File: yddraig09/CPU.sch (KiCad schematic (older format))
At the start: 4 parts

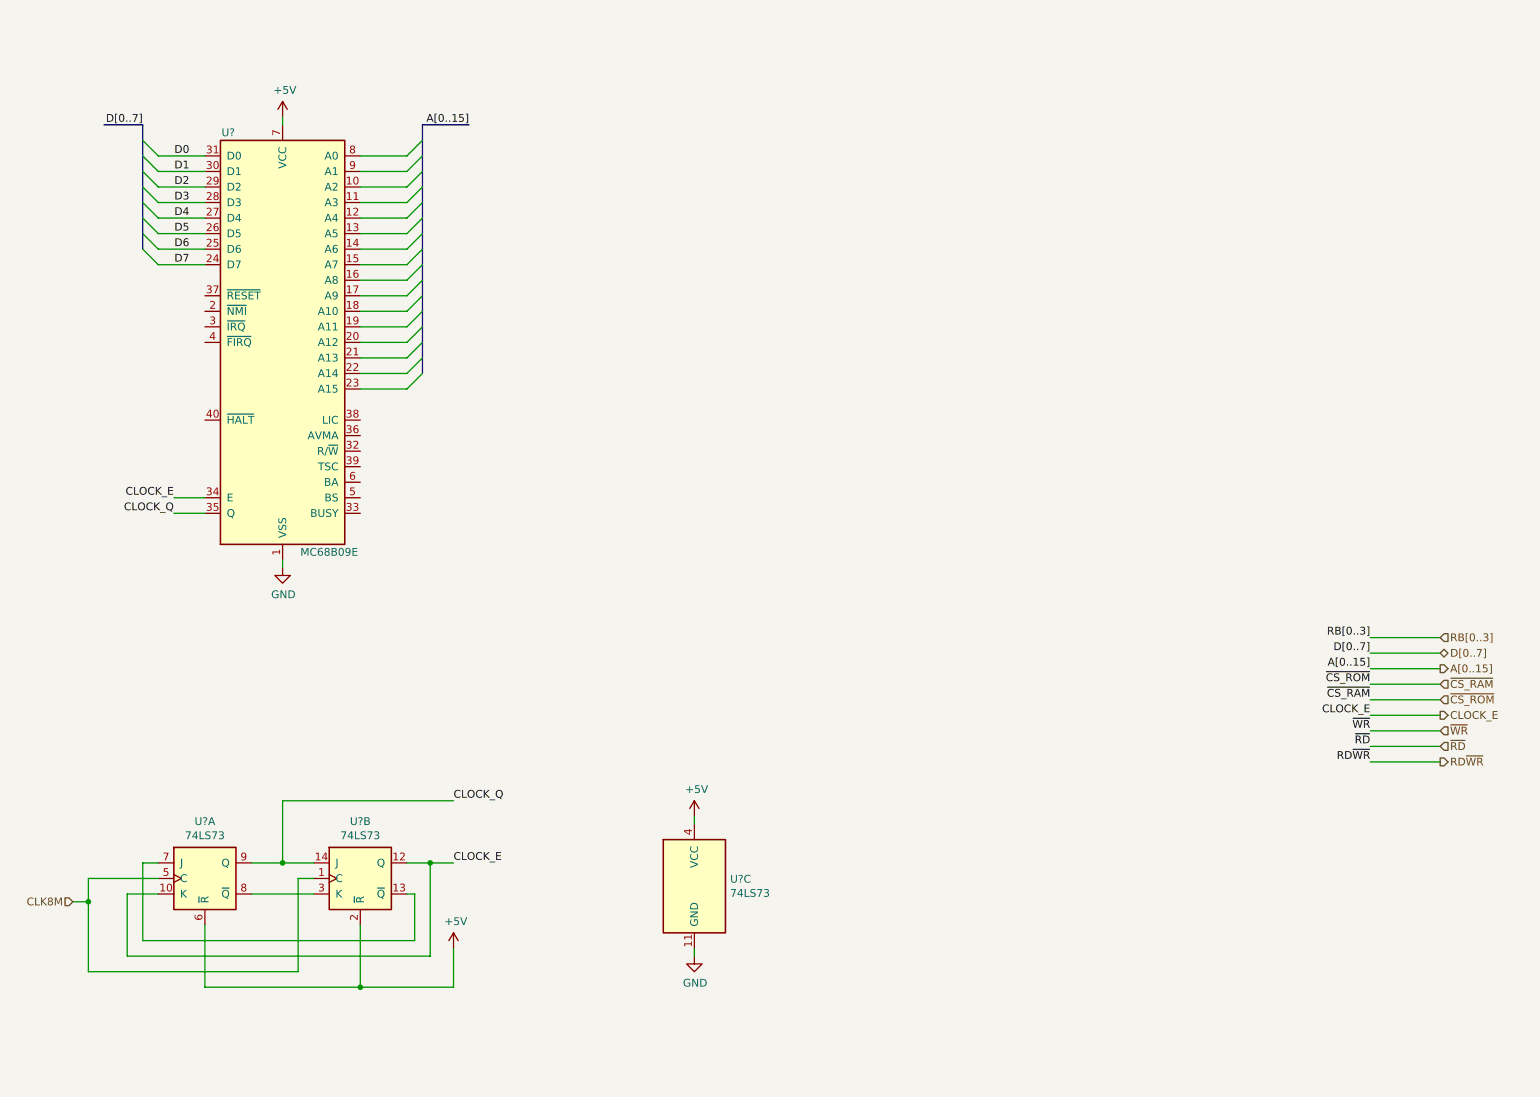
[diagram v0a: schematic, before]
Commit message: Some tidying up of 6809 project
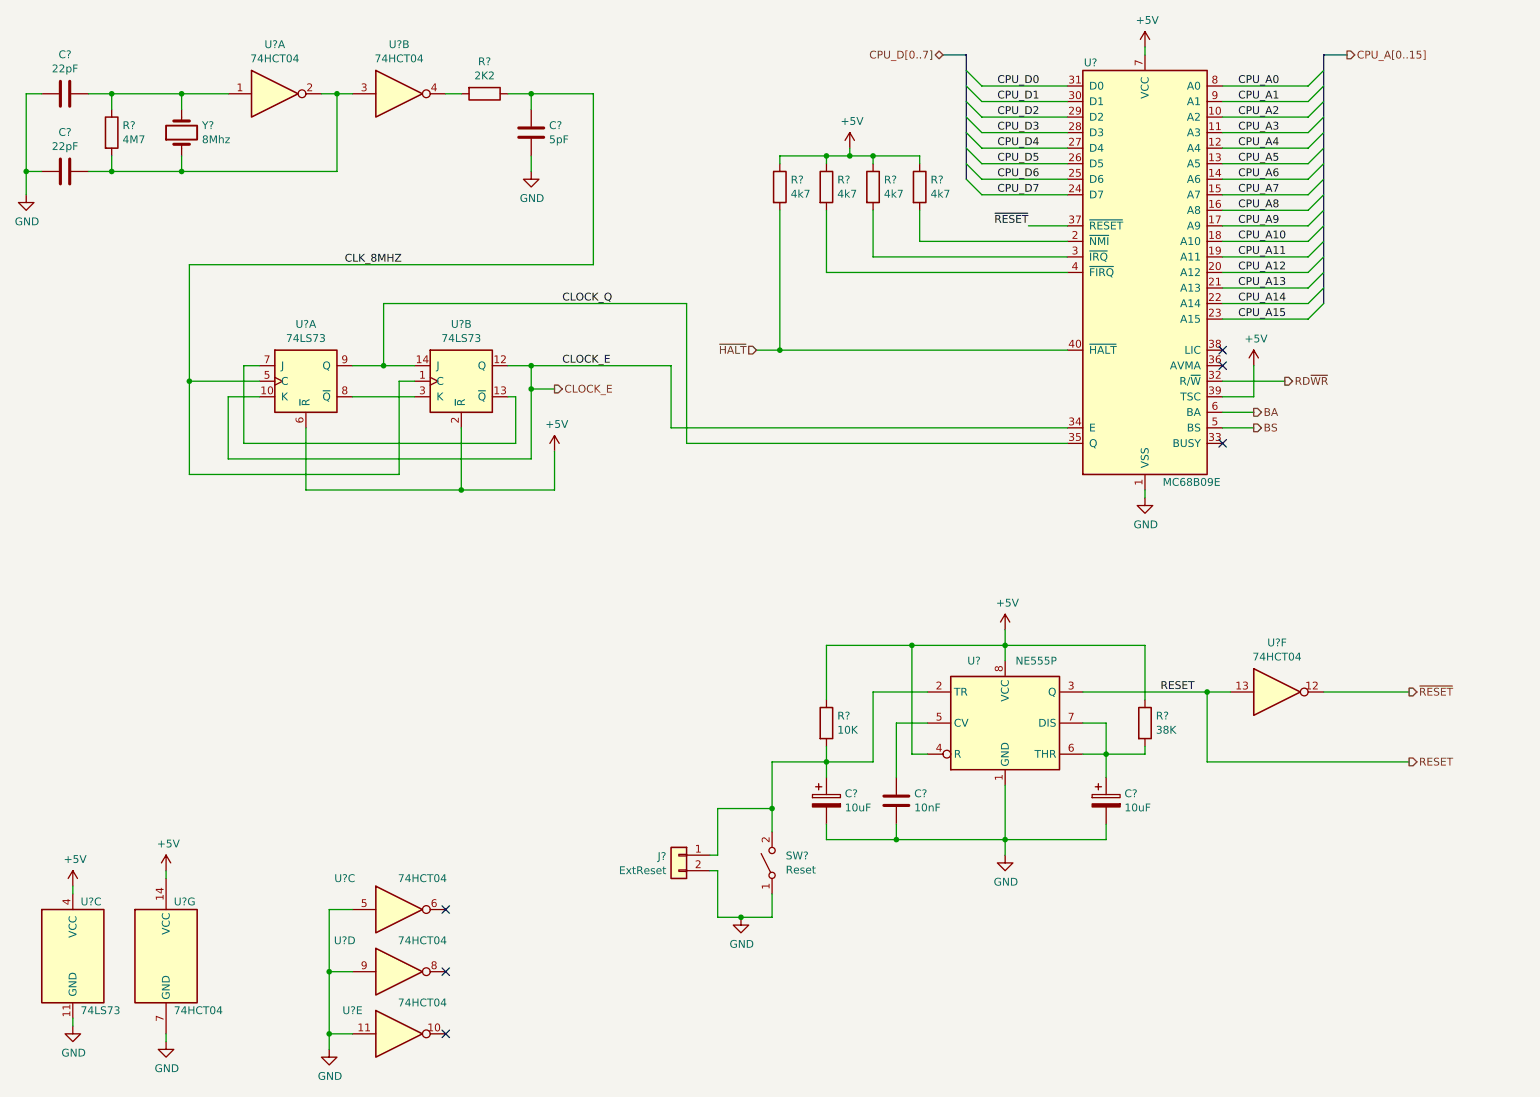
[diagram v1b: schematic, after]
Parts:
- added C? (x2): 10uF, Capacitor_THT:CP_Radial_D5.0mm_P2.50mm, symbol Device:CP
- added C?: 10nF, Capacitor_THT:C_Disc_D3.8mm_W2.6mm_P2.50mm, symbol Device:C
- added C? (x2): 22pF, Capacitor_THT:C_Disc_D5.0mm_W2.5mm_P2.50mm, symbol Device:C
- added C?: 5pF, Capacitor_THT:C_Disc_D5.0mm_W2.5mm_P2.50mm, symbol Device:C
- added J?: ExtReset, Connector_PinHeader_2.54mm:PinHeader_1x02_P2.54mm_Vertical, symbol Connector_Generic:Conn_01x02
- added R?: 10K, Resistor_THT:R_Axial_DIN0207_L6.3mm_D2.5mm_P10.16mm_Horizontal, symbol Device:R
- added R?: 38K, Resistor_THT:R_Axial_DIN0207_L6.3mm_D2.5mm_P10.16mm_Horizontal, symbol Device:R
- added R? (x4): 4k7, symbol Device:R
- added R?: 4M7, Resistor_THT:R_Axial_DIN0207_L6.3mm_D2.5mm_P10.16mm_Horizontal, symbol Device:R
- added R?: 2K2, Resistor_THT:R_Axial_DIN0207_L6.3mm_D2.5mm_P10.16mm_Horizontal, symbol Device:R
- added SW?: Reset, Button_Switch_THT:SW_PUSH_6mm_H4.3mm, symbol Switch:SW_SPST
- added U?: NE555P, Package_DIP:DIP-8_W7.62mm, symbol Timer:NE555P
- added U? (x7): 74HCT04, symbol 74xx:74HCT04
- added Y?: 8Mhz, Crystal:Crystal_HC50_Vertical, symbol Device:Crystal
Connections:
- net +5V: now also U?.39 (TSC), R?.1, R?.1, R?.1, R?.1, R?.1, R?.1, U?.14 (VCC), U?.4 (R), U?.8 (VCC)
- net GND: now also C?.2, C?.2, C?.2, C?.2, C?.2, C?.2, J?.2 (Pin_2), SW?.1 (A), U?.1 (GND), U?.11, U?.5, U?.7 (GND), U?.9
- net RD~WR: now also U?.32 (R/~W)
- net CPU_A2: now reaches U?.10 (A2)
- net CPU_A3: now reaches U?.11 (A3)
- net CPU_A4: now reaches U?.12 (A4)
- net CPU_A5: now reaches U?.13 (A5)
- net CPU_A6: now reaches U?.14 (A6)
- net CPU_A7: now reaches U?.15 (A7)
- net CPU_A8: now reaches U?.16 (A8)
- net CPU_A9: now reaches U?.17 (A9)
- net CPU_A10: now reaches U?.18 (A10)
- net CPU_A11: now reaches U?.19 (A11)
- net at U?.2 (~NMI): now also R?.2
- net CPU_A12: now reaches U?.20 (A12)
- net CPU_A13: now reaches U?.21 (A13)
- net CPU_A14: now reaches U?.22 (A14)
- net CPU_A15: now reaches U?.23 (A15)
- net at U?.3 (~IRQ): now also R?.2
- net ~RESET: now reaches U?.37 (~RESET)
- net ~RESET: now also U?.12
- net at U?.4 (~FIRQ): now also R?.2
- net ~HALT: now reaches U?.40 (~HALT)
- net ~HALT: now also R?.2
- net BS: now reaches U?.5 (BS)
- net BA: now reaches U?.6 (BA)
- net CPU_A0: now reaches U?.8 (A0)
- net CPU_A1: now reaches U?.9 (A1)
- net CLK8M renamed CLK_8MHZ
- net CLK_8MHZ: now also C?.1, R?.1
- net D0 renamed CPU_D0
- net D1 renamed CPU_D1
- net D2 renamed CPU_D2
- net D3 renamed CPU_D3
- net D4 renamed CPU_D4
- net D5 renamed CPU_D5
- net D6 renamed CPU_D6
- net D7 renamed CPU_D7
- new net: C?.1, J?.1 (Pin_1), R?.2, SW?.2 (B), U?.2 (TR)
- new net: C?.1, U?.5 (CV)
- new net: C?.1, R?.2, U?.6 (THR), U?.7 (DIS)
- new net: C?.1, R?.1, U?.1, Y?.2
- new net: C?.1, R?.2, U?.2, U?.3, Y?.1
- new net: R?.2, U?.4
- new net RESET: U?.13, U?.3 (Q)
- no-connect marks 0 -> 6
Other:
- moved on the sheet: U?, U?A, U?B, U?C

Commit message: more progress
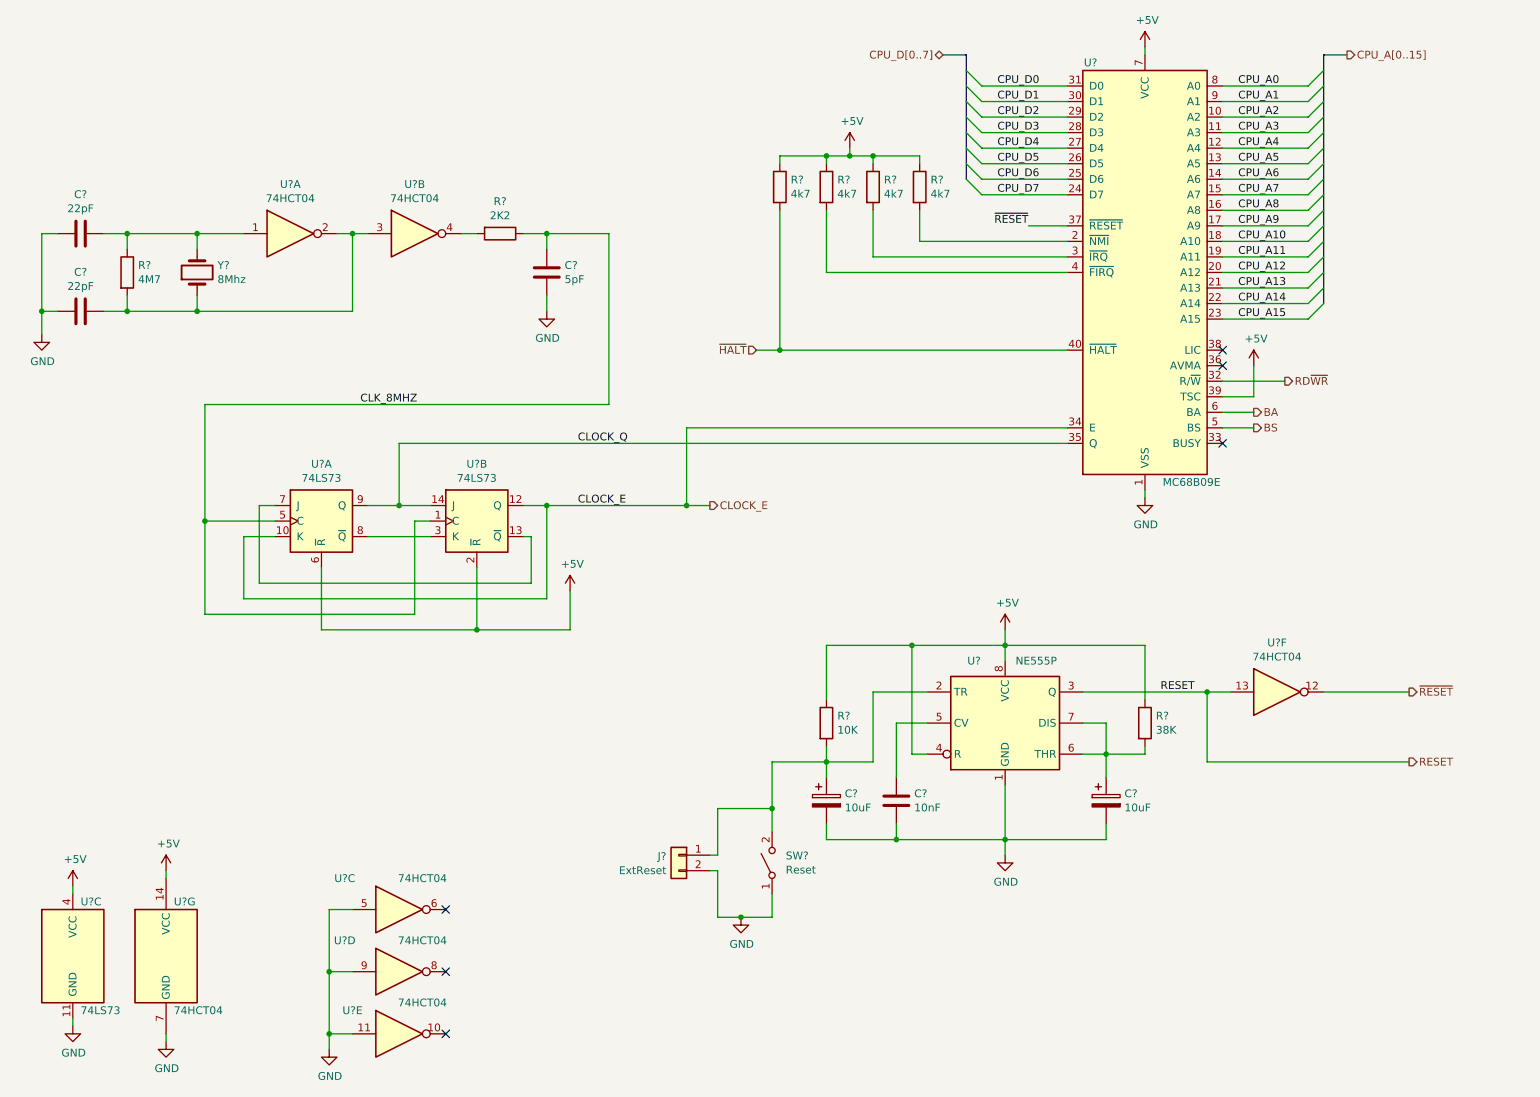
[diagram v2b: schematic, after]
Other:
- moved on the sheet: C?, R?, U?A, U?B, Y?
